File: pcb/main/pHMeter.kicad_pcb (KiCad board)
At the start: 2 copper layers, 100 x 87 mm, 147 parts, among them J1 Conn_02x03_Odd_Even, J2 Conn_Coaxial_Power, J3 Conn_Coaxial_Power, J4 AudioJack3_SwitchTR, J5 RJ12, J6 AudioJack3_SwitchTR, J7 SJ, J8 SJ, Q1 ZXMS6004, Q2 ZXMS6004, Q3 DMP1045, Q4 ZXMS6004, Q5 ZXMS6004, SW1 Rotary_Encoder_Switch, U1 TLV6004PW, U2 TLV6004PW, U3 ATMEGA32U4-AU, U4 MCP1703A, U5 AP63203WU-7, U6 HX711, U7 SST26VF064B, U9 MCP73811T, X1 MINI-USB-SCHIELD-32005-201, Y1 Crystal

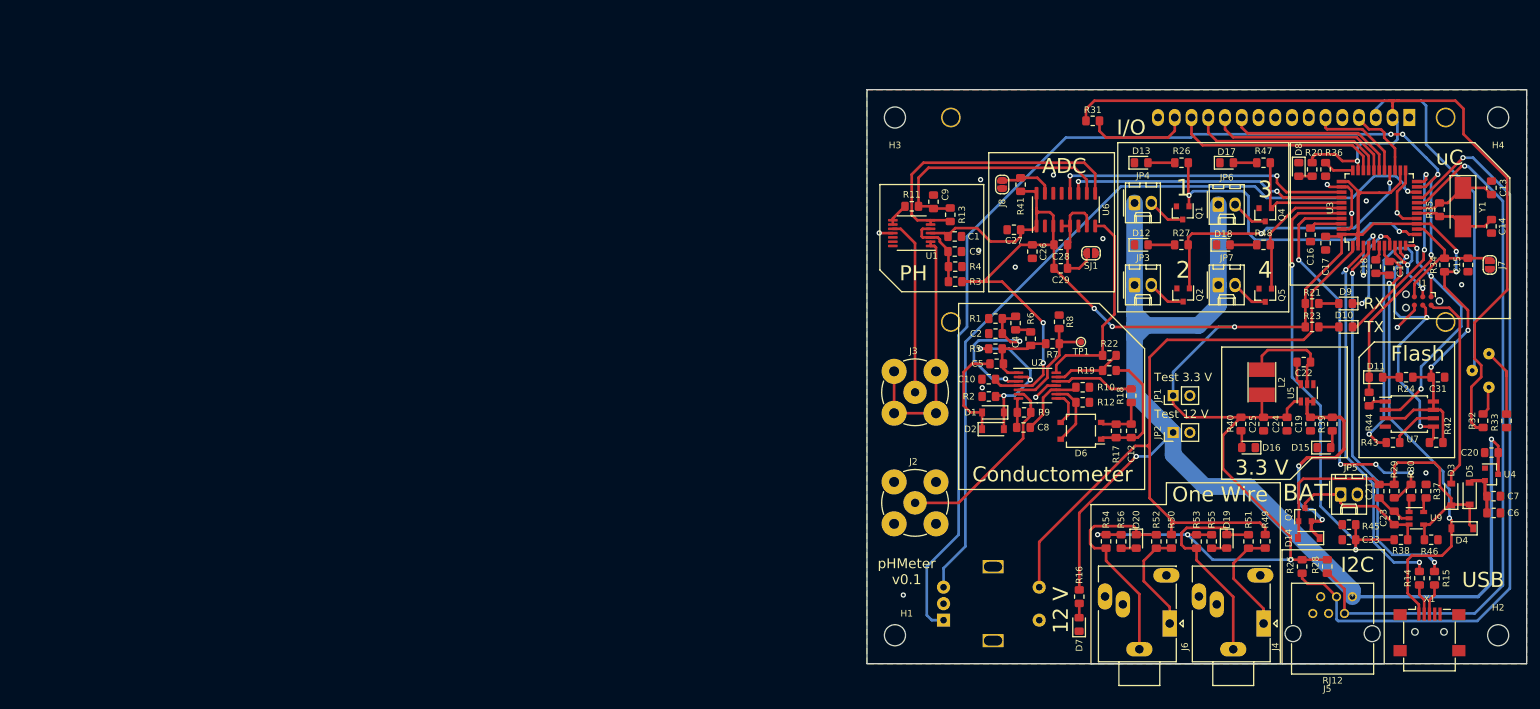
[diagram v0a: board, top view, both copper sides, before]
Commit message: fix: refactor hardware design
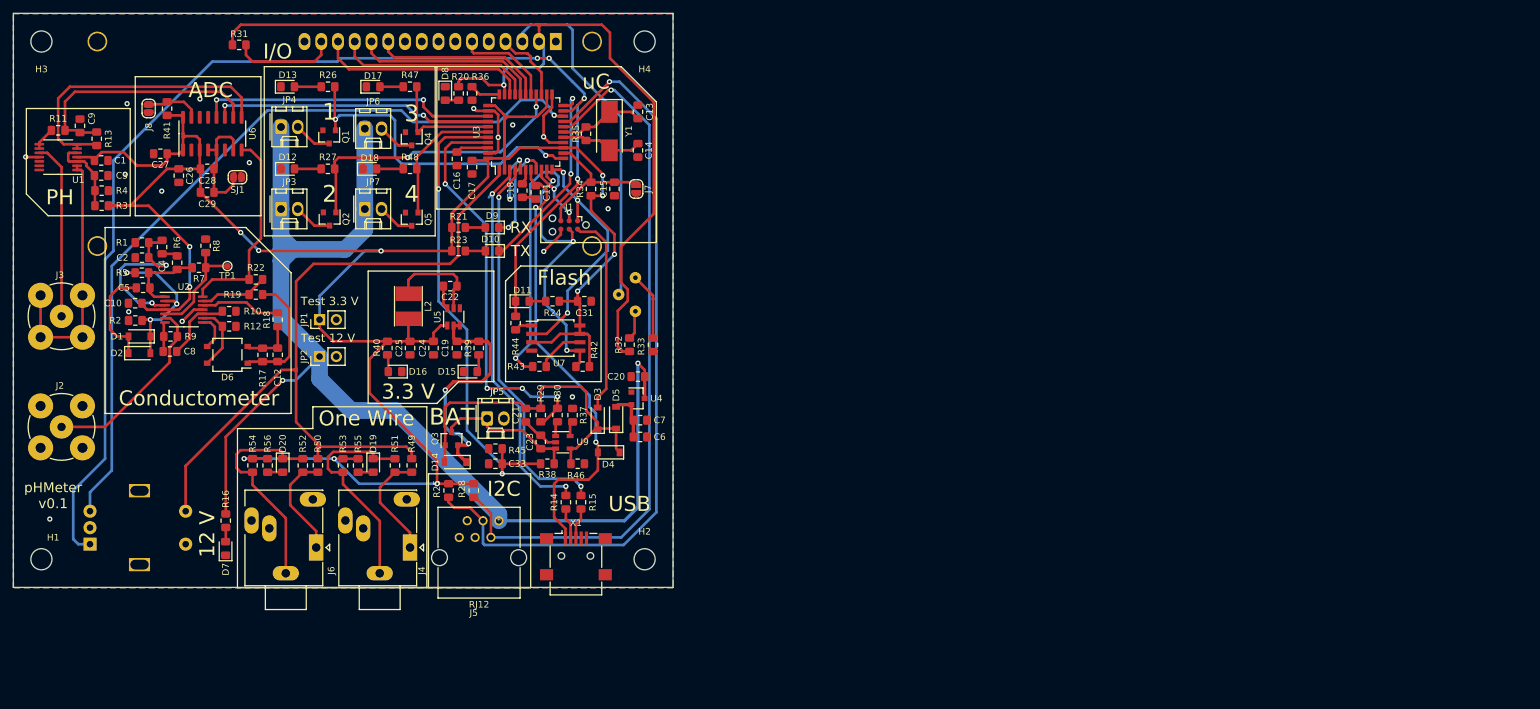
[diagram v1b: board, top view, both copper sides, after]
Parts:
- moved D4 129.9 mm to (140.3, 116.5)
- moved C1 129.9 mm to (63.3, 72.3)
- moved C10 129.9 mm to (68.5, 93.9)
- moved C11 129.9 mm to (129.2, 77.1)
- moved C18 129.9 mm to (127.2, 76.9)
- moved C21 129.9 mm to (127.7, 110.9)
- moved C22 129.9 mm to (116.2, 91.4)
- moved C23 129.9 mm to (129.9, 115.0)
- moved C24 129.9 mm to (113.7, 100.7)
- moved C26 129.9 mm to (75.1, 74.6)
- moved C28 129.9 mm to (79.4, 73.6)
- moved C29 129.9 mm to (79.4, 77.1)
- moved C3 129.9 mm to (63.3, 74.6)
- moved C31 129.9 mm to (136.6, 93.6)
- moved C33 129.9 mm to (123.1, 118.3)
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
